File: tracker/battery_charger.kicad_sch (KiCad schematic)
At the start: 17 parts, among them Q3 SSM6N7002KFU, U8 BQ25601

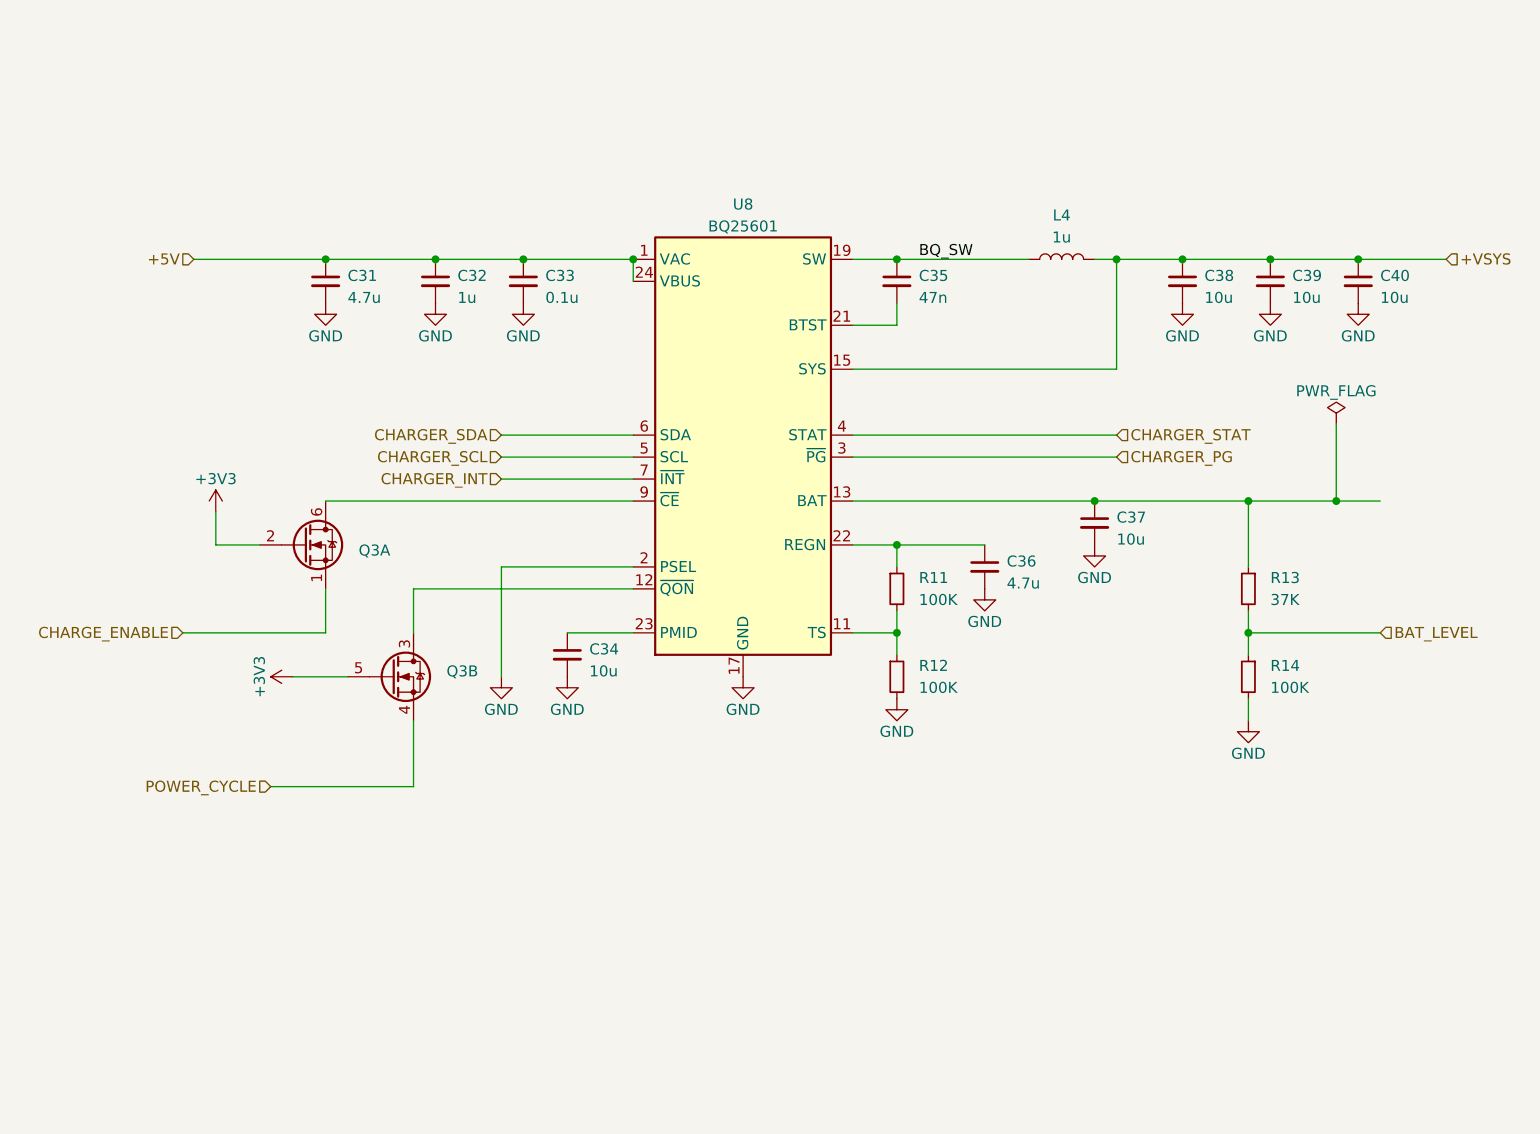
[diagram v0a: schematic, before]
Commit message: first version
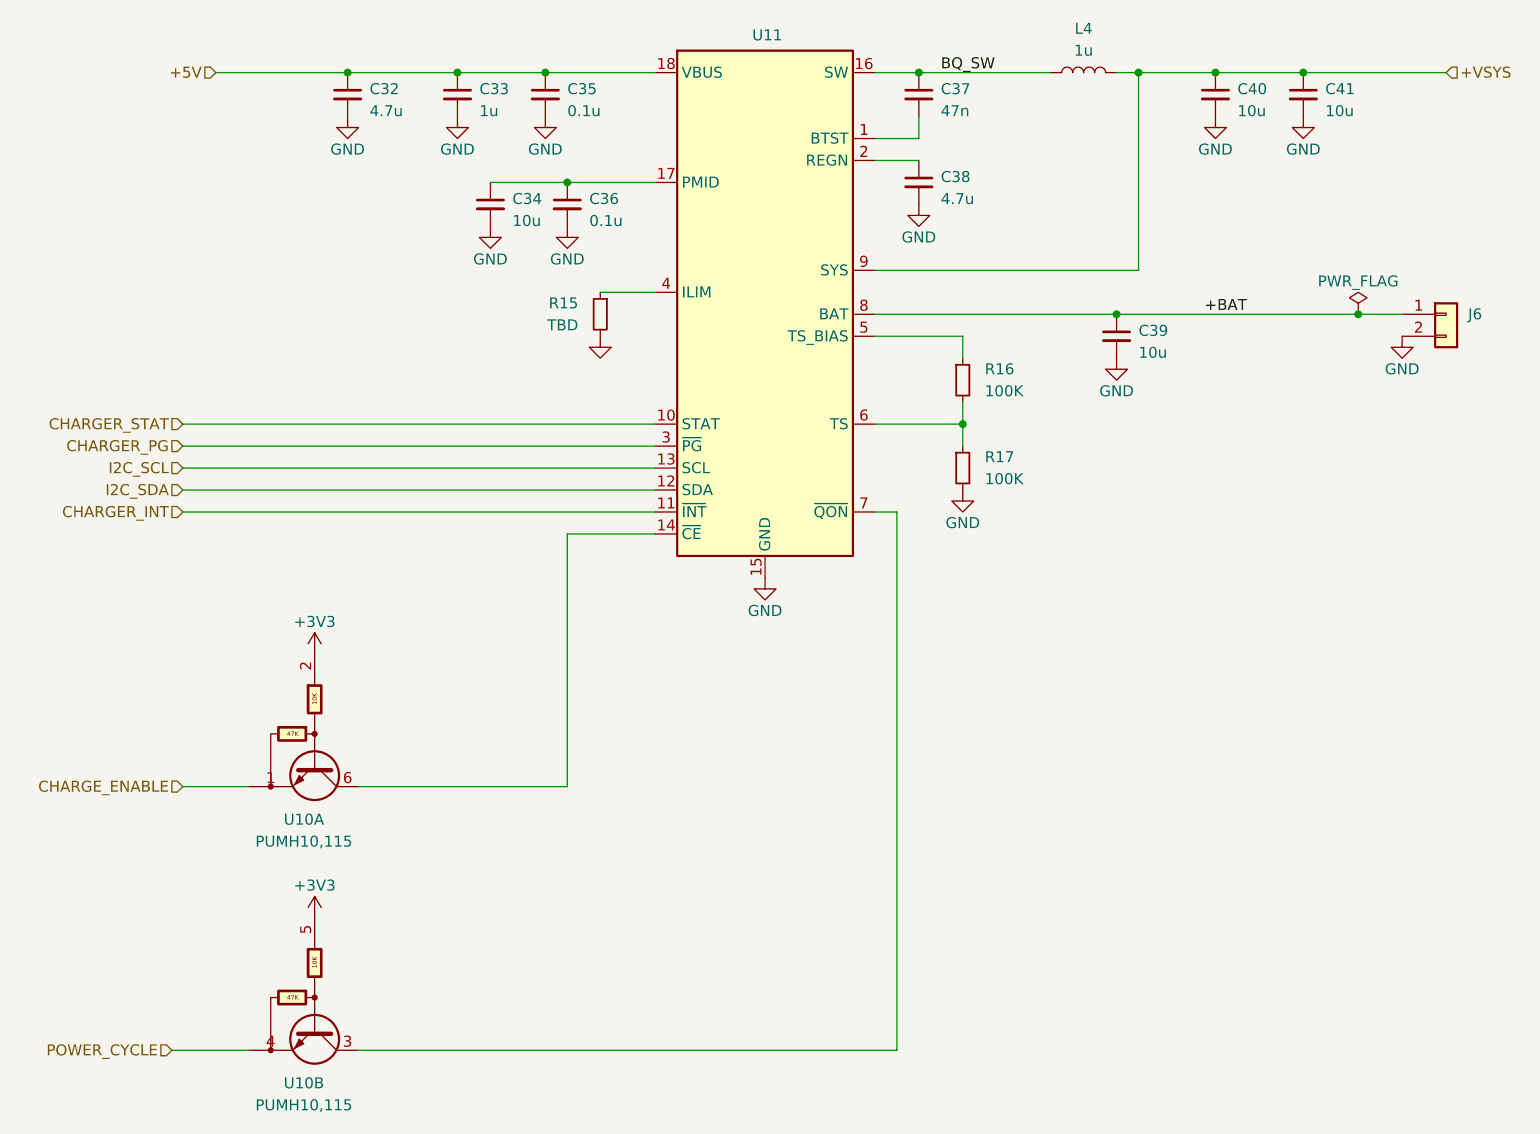
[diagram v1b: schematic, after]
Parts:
- removed C38: 10u, Capacitor_SMD:C_0805_2012Metric, symbol Device:C_Small
- removed Q3: SSM6N7002KFU, Package_TO_SOT_SMD:SOT-363_SC-70-6, symbol Device:Q_Dual_NMOS_S1G1D2S2G2D1
- removed R13: 37K, Resistor_SMD:R_0402_1005Metric, symbol Device:R_Small
- removed R14: 100K, Resistor_SMD:R_0402_1005Metric, symbol Device:R_Small
- removed U8: BQ25601, Package_DFN_QFN:Texas_RTW_WQFN-24-1EP_4x4mm_P0.5mm_EP2.7x2.7mm_ThermalVias, symbol Battery_Management:BQ25601
- added C36: 0.1u, Capacitor_SMD:C_0603_1608Metric, symbol Device:C_Small
- added J6: Conn_01x02, Connector_JST:JST_XH_B2B-XH-A_1x02_P2.50mm_Vertical, symbol Connector_Generic:Conn_01x02
- added R15: TBD, Resistor_SMD:R_0402_1005Metric, symbol Device:R_Small
- added U10: PUMH10,115, Package_TO_SOT_SMD:SOT-363_SC-70-6, symbol My Libraries:PUMH10,115
- added U11: ~, My Footprints:BQ25622E, symbol My Libraries:BQ25622E
- renumbered C31 to C32, C32 to C33, C33 to C35, C35 to C37, C36 to C38, C37 to C39, C39 to C40, C40 to C41, R11 to R16, R12 to R17
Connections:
- net +3V3: now also U10.2, U10.5
- net +5V: now also U11.18 (VBUS)
- net +VSYS: now also U11.9 (SYS)
- net BQ_SW: now also U11.16 (SW)
- net CHARGER_INT: now also U11.11 (~{INT})
- net CHARGER_PG: now also U11.3 (~{PG})
- net CHARGER_STAT: now also U11.10 (STAT)
- net CHARGE_ENABLE: now also U10.1
- net GND: now also C36.2, J6.2 (Pin_2), R15.2, U11.15 (GND)
- net POWER_CYCLE: now also U10.4
- net at C37.2: now also U11.1 (BTST)
- net +BAT: now reaches C39.1
- net +BAT: now also J6.1 (Pin_1), U11.8 (BAT)
- net at C34.1: now also C36.1, U11.17 (PMID)
- net at C38.1: now also U11.2 (REGN); no longer R16.1
- net at R16.2, R17.1: now also U11.6 (TS)
- new net: U10.6, U11.14 (~{CE})
- new net: R15.1, U11.4 (ILIM)
- new net: R16.1, U11.5 (TS_BIAS)
- new net: U10.3, U11.7 (~{QON})
- new net I2C_SCL: U11.13 (SCL)
- new net I2C_SDA: U11.12 (SDA)
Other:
- moved on the sheet: C32, C33, C35, C37, C38, C39, C40, C41, L4, R16, R17
